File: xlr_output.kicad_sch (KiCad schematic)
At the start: 5 parts, among them J1 XLR3, J2 XLR3, J3 XLR3, J4 XLR3, SW1 SW_SPDT

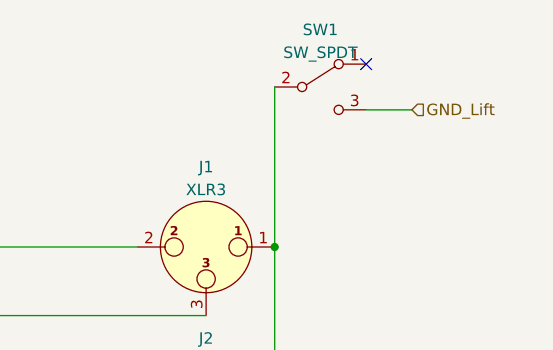
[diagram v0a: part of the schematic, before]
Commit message: Small fixes, schmeatic complete
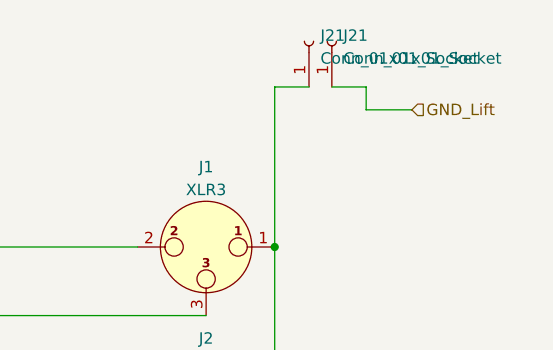
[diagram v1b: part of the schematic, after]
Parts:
- removed SW1: SW_SPDT, symbol Switch:SW_SPDT
- added J21 (x2): Conn_01x01_Socket, Connector_Wire:SolderWire-0.75sqmm_1x01_D1.25mm_OD2.3mm, symbol Connector:Conn_01x01_Socket
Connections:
- net GND_Lift: now also J21.1 (Pin_1)
- net at J1.1, J2.1, J3.1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: now also J21.1 (Pin_1)
- no-connect marks 1 -> 0
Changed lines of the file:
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@@
   (junction (at 163.83 92.71) (diameter 0) (color 0 0 0 0)
   )
-  (no_connect (at 173.99 53.34))
   (wire (pts (xy 156.21 119.38) (xy 123.19 119.38))
     (stroke (width 0) (type default))
   )
+  (wire (pts (xy 173.99 55.88) (xy 173.99 58.42))
+    (stroke (width 0) (type default))
+  )
   (wire (pts (xy 173.99 58.42) (xy 179.07 58.42))
     (stroke (width 0) (type default))
@@
   )
   (wire (pts (xy 148.59 111.76) (xy 123.19 111.76))
+    (stroke (width 0) (type default))
+  )
+  (wire (pts (xy 170.18 55.88) (xy 173.99 55.88))
+    (stroke (width 0) (type default))
+  )
+  (wire (pts (xy 163.83 55.88) (xy 167.64 55.88))
     (stroke (width 0) (type default))
   )
@@
     )
   )
-  (symbol (lib_id "Switch:SW_SPDT") (at 168.91 55.88 0) (unit 1)
-    (in_bom yes) (on_board yes) (dnp no)
-    (property "Reference" "SW1" (at 168.91 49.53 0)
-      (effects (font (size 1.27 1.27)))
-    )
-    (property "Value" "SW_SPDT" (at 168.91 52.07 0)
-      (effects (font (size 1.27 1.27)))
-    )
-    (property "Footprint" "" (at 168.91 55.88 0)
-      (effects (font (size 1.27 1.27)) hide)
-    )
-    (property "Datasheet" "~" (at 168.91 55.88 0)
+  (symbol (lib_id "Connector_Audio:XLR3") (at 156.21 130.81 0) (mirror y) (unit 1)
+    (in_bom yes) (on_board yes) (dnp no) (fields_autoplaced)
+    (property "Reference" "J4" (at 156.21 121.92 0)
+      (effects (font (size 1.27 1.27)))
+    )
+    (property "Value" "XLR3" (at 156.21 124.46 0)
+      (effects (font (size 1.27 1.27)))
+    )
+    (property "Footprint" "" (at 156.21 130.81 0)
+      (effects (font (size 1.27 1.27)) hide)
+    )
+    (property "Datasheet" " ~" (at 156.21 130.81 0)
       (effects (font (size 1.27 1.27)) hide)
     )
@@
       (project "EF_matrix"
         (path "/621f65ee-d66d-40b7-9a89-3052b9373190"
-          (reference "SW1") (unit 1)
-        )
-        (path "/621f65ee-d66d-40b7-9a89-3052b9373190/837cbbaa-ad41-4de8-bb02-f85faf12da13"
-          (reference "SW2") (unit 1)
-        )
-        (path "/621f65ee-d66d-40b7-9a89-3052b9373190/64851fbd-c688-4197-a63d-3dce17468ba2"
-          (reference "SW3") (unit 1)
-        )
-        (path "/621f65ee-d66d-40b7-9a89-3052b9373190/d94772af-2feb-48c7-98be-bb0e397012c8"
-          (reference "SW4") (unit 1)
-        )
-      )
-    )
-  )
-  (symbol (lib_id "Connector_Audio:XLR3") (at 156.21 130.81 0) (mirror y) (unit 1)
-    (in_bom yes) (on_board yes) (dnp no) (fields_autoplaced)
-    (property "Reference" "J4" (at 156.21 121.92 0)
-      (effects (font (size 1.27 1.27)))
-    )
-    (property "Value" "XLR3" (at 156.21 124.46 0)
-      (effects (font (size 1.27 1.27)))
-    )
-    (property "Footprint" "" (at 156.21 130.81 0)
-      (effects (font (size 1.27 1.27)) hide)
-    )
-    (property "Datasheet" " ~" (at 156.21 130.81 0)
+          (reference "J4") (unit 1)
+        )
+        (path "/621f65ee-d66d-40b7-9a89-3052b9373190/837cbbaa-ad41-4de8-bb02-f85faf12da13"
+          (reference "J8") (unit 1)
+        )
+        (path "/621f65ee-d66d-40b7-9a89-3052b9373190/64851fbd-c688-4197-a63d-3dce17468ba2"
+          (reference "J12") (unit 1)
+        )
+        (path "/621f65ee-d66d-40b7-9a89-3052b9373190/d94772af-2feb-48c7-98be-bb0e397012c8"
+          (reference "J16") (unit 1)
+        )
+      )
+    )
+  )
+  (symbol (lib_id "Connector_Audio:XLR3") (at 156.21 111.76 0) (mirror y) (unit 1)
+    (in_bom yes) (on_board yes) (dnp no) (fields_autoplaced)
+    (property "Reference" "J3" (at 156.21 102.87 0)
+      (effects (font (size 1.27 1.27)))
+    )
+    (property "Value" "XLR3" (at 156.21 105.41 0)
+      (effects (font (size 1.27 1.27)))
+    )
+    (property "Footprint" "" (at 156.21 111.76 0)
+      (effects (font (size 1.27 1.27)) hide)
+    )
+    (property "Datasheet" " ~" (at 156.21 111.76 0)
       (effects (font (size 1.27 1.27)) hide)
     )
@@
       (project "EF_matrix"
         (path "/621f65ee-d66d-40b7-9a89-3052b9373190"
-          (reference "J4") (unit 1)
-        )
-        (path "/621f65ee-d66d-40b7-9a89-3052b9373190/837cbbaa-ad41-4de8-bb02-f85faf12da13"
-          (reference "J8") (unit 1)
-        )
-        (path "/621f65ee-d66d-40b7-9a89-3052b9373190/64851fbd-c688-4197-a63d-3dce17468ba2"
-          (reference "J12") (unit 1)
-        )
-        (path "/621f65ee-d66d-40b7-9a89-3052b9373190/d94772af-2feb-48c7-98be-bb0e397012c8"
-          (reference "J16") (unit 1)
-        )
-      )
-    )
-  )
-  (symbol (lib_id "Connector_Audio:XLR3") (at 156.21 111.76 0) (mirror y) (unit 1)
-    (in_bom yes) (on_board yes) (dnp no) (fields_autoplaced)
-    (property "Reference" "J3" (at 156.21 102.87 0)
-      (effects (font (size 1.27 1.27)))
-    )
-    (property "Value" "XLR3" (at 156.21 105.41 0)
-      (effects (font (size 1.27 1.27)))
-    )
-    (property "Footprint" "" (at 156.21 111.76 0)
-      (effects (font (size 1.27 1.27)) hide)
-    )
-    (property "Datasheet" " ~" (at 156.21 111.76 0)
-      (effects (font (size 1.27 1.27)) hide)
-    )
-    (pin "1")
-    (pin "2")
-    (pin "3")
-    (instances
-      (project "EF_matrix"
-        (path "/621f65ee-d66d-40b7-9a89-3052b9373190"
           (reference "J3") (unit 1)
         )
@@
         )
       )
+    )
+  )
+  (symbol (lib_id "Connector:Conn_01x01_Socket") (at 170.18 50.8 90) (unit 1)
+    (in_bom yes) (on_board yes) (dnp no) (fields_autoplaced)
+    (property "Reference" "J21" (at 171.45 50.165 90)
+      (effects (font (size 1.27 1.27)) (justify right))
+    )
+    (property "Value" "Conn_01x01_Socket" (at 171.45 52.705 90)
+      (effects (font (size 1.27 1.27)) (justify right))
+    )
+    (property "Footprint" "Connector_Wire:SolderWire-0.75sqmm_1x01_D1.25mm_OD2.3mm" (at 170.18 50.8 0)
+      (effects (font (size 1.27 1.27)) hide)
+    )
+    (property "Datasheet" "~" (at 170.18 50.8 0)
+      (effects (font (size 1.27 1.27)) hide)
+    )
+    (pin "1")
+    (instances
+      (project "EF_matrix"
+        (path "/621f65ee-d66d-40b7-9a89-3052b9373190/b97d10d9-dc84-4d90-b1cc-f43ccd4b156b"
+          (reference "J21") (unit 1)
+        )
+        (path "/621f65ee-d66d-40b7-9a89-3052b9373190/837cbbaa-ad41-4de8-bb02-f85faf12da13"
+          (reference "J25") (unit 1)
+        )
+        (path "/621f65ee-d66d-40b7-9a89-3052b9373190/64851fbd-c688-4197-a63d-3dce17468ba2"
+          (reference "J26") (unit 1)
+        )
+        (path "/621f65ee-d66d-40b7-9a89-3052b9373190/d94772af-2feb-48c7-98be-bb0e397012c8"
+          (reference "J34") (unit 1)
+        )
+      )
+    )
+  )
+  (symbol (lib_id "Connector:Conn_01x01_Socket") (at 167.64 50.8 90) (unit 1)
+    (in_bom yes) (on_board yes) (dnp no) (fields_autoplaced)
+    (property "Reference" "J21" (at 168.91 50.165 90)
+      (effects (font (size 1.27 1.27)) (justify right))
+    )
+    (property "Value" "Conn_01x01_Socket" (at 168.91 52.705 90)
+      (effects (font (size 1.27 1.27)) (justify right))
+    )
+    (property "Footprint" "Connector_Wire:SolderWire-0.75sqmm_1x01_D1.25mm_OD2.3mm" (at 167.64 50.8 0)
+      (effects (font (size 1.27 1.27)) hide)
+    )
+    (property "Datasheet" "~" (at 167.64 50.8 0)
+      (effects (font (size 1.27 1.27)) hide)
+    )
+    (pin "1")
+    (instances
+      (project "EF_matrix"
+        (path "/621f65ee-d66d-40b7-9a89-3052b9373190/b97d10d9-dc84-4d90-b1cc-f43ccd4b156b"
+          (reference "J21") (unit 1)
+        )
+        (path "/621f65ee-d66d-40b7-9a89-3052b9373190/837cbbaa-ad41-4de8-bb02-f85faf12da13"
+          (reference "J22") (unit 1)
+        )
+        (path "/621f65ee-d66d-40b7-9a89-3052b9373190/64851fbd-c688-4197-a63d-3dce17468ba2"
+          (reference "J23") (unit 1)
+        )
+        (path "/621f65ee-d66d-40b7-9a89-3052b9373190/d94772af-2feb-48c7-98be-bb0e397012c8"
+          (reference "J2") (unit 1)
+        )
+      )
